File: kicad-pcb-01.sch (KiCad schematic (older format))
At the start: 24 parts, among them SW1 SW_Push, U1 ATmega32U4-AU, Y1 16MHz

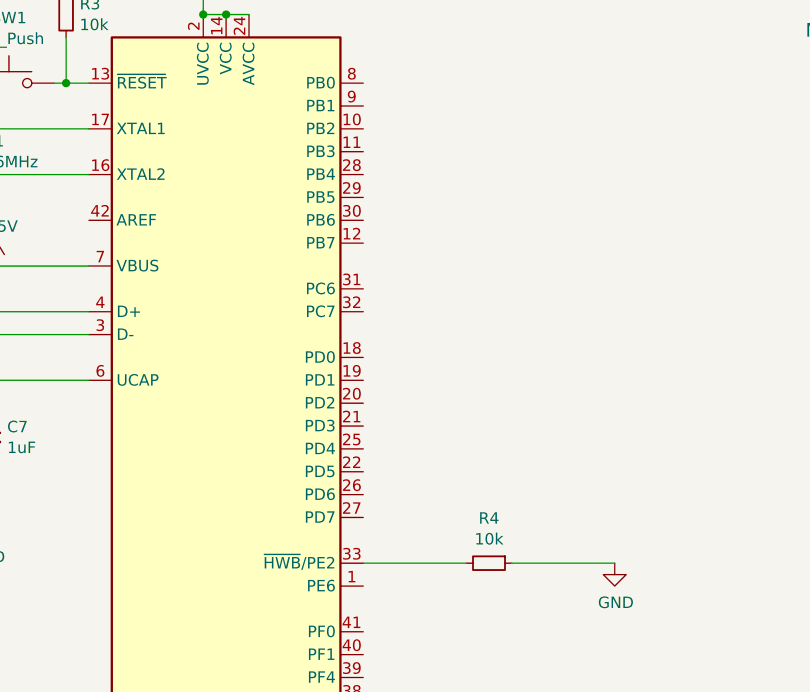
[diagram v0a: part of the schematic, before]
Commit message: routing complete
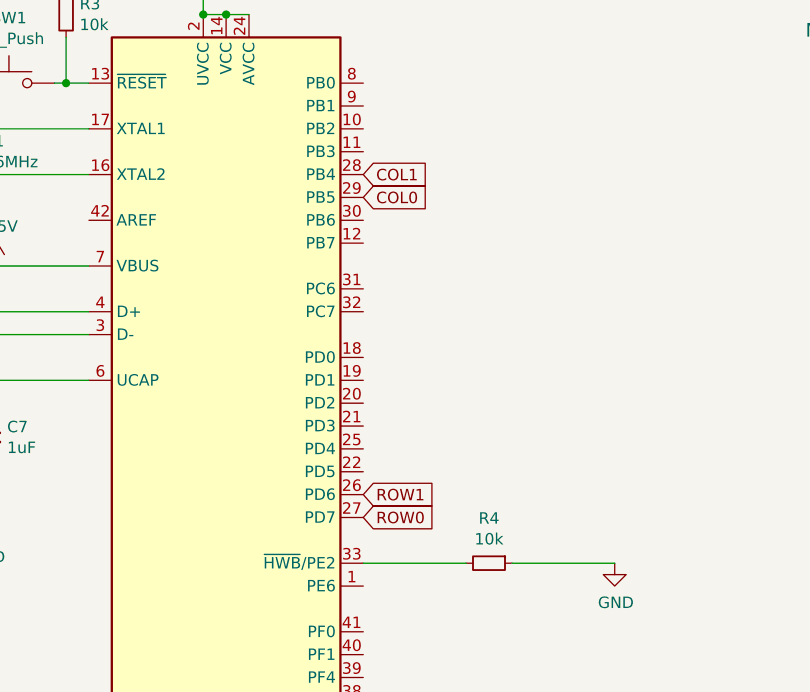
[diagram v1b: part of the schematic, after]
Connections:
- net COL0: now also U1.29 (PB5)
- net COL1: now also U1.28 (PB4)
- net ROW0: now also U1.27 (PD7)
- net ROW1: now also U1.26 (PD6)
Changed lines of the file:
@@
 Text GLabel 8050 2500 1    50   Input ~ 0
 COL1
+Text GLabel 4050 3150 2    50   Input ~ 0
+ROW1
+Text GLabel 4050 3250 2    50   Input ~ 0
+ROW0
+Text GLabel 4050 1750 2    50   Input ~ 0
+COL1
+Text GLabel 4050 1850 2    50   Input ~ 0
+COL0
 $EndSCHEMATC

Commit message: added lcsc part ref:
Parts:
- C1, C2, C3: LCSC (none) -> C1711
- C4, C5: LCSC (none) -> C465168
- C6: LCSC (none) -> C307520
- C7: LCSC (none) -> C116352
- D1, D2, D3, D4: LCSC (none) -> C77978
- F1: LCSC (none) -> C151162
- R1, R2: LCSC (none) -> C413152
- R3, R4: LCSC (none) -> C191101
- SW1: LCSC (none) -> C221929
- U1: LCSC (none) -> C44854
- USB1: LCSC (none) -> C105424
- Y1: LCSC (none) -> C254367
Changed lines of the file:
@@
 F 2 "Package_QFP:TQFP-44_10x10mm_P0.8mm" H 3450 2850 50  0001 C CIN
 F 3 "http://ww1.microchip.com/downloads/en/DeviceDoc/Atmel-7766-8-bit-AVR-ATmega16U4-32U4_Datasheet.pdf" H 3450 2850 50  0001 C CNN
+F 4 "C44854" H 3450 2850 50  0001 C CNN "LCSC"
 	1    3450 2850
 	1    0    0    -1
@@
 F 2 "Resistor_SMD:R_0805_2012Metric" H 4600 3450 50  0001 C CNN
 F 3 "~" H 4600 3450 50  0001 C CNN
+F 4 "C191101" V 4600 3450 50  0001 C CNN "LCSC"
 	1    4600 3450
 	0    1    1    0
@@
 F 2 "Resistor_SMD:R_0805_2012Metric" H 2300 2350 50  0001 C CNN
 F 3 "~" H 2300 2350 50  0001 C CNN
+F 4 "C413152" V 2300 2350 50  0001 C CNN "LCSC"
 	1    2300 2350
 	0    1    1    0
@@
 F 2 "Resistor_SMD:R_0805_2012Metric" H 2000 2450 50  0001 C CNN
 F 3 "~" H 2000 2450 50  0001 C CNN
+F 4 "C413152" V 2000 2450 50  0001 C CNN "LCSC"
 	1    2000 2450
 	0    1    1    0
@@
 F 2 "Capacitor_SMD:C_0805_2012Metric" H 2400 2900 50  0001 C CNN
 F 3 "~" H 2400 2900 50  0001 C CNN
+F 4 "C116352" H 2400 2900 50  0001 C CNN "LCSC"
 	1    2400 2900
 	1    0    0    -1
@@
 F 2 "Capacitor_SMD:C_0805_2012Metric" H 850 4050 50  0001 C CNN
 F 3 "~" H 850 4050 50  0001 C CNN
+F 4 "C1711" H 850 4050 50  0001 C CNN "LCSC"
 	1    850  4050
 	1    0    0    -1
@@
 F 2 "Capacitor_SMD:C_0805_2012Metric" H 1300 4050 50  0001 C CNN
 F 3 "~" H 1300 4050 50  0001 C CNN
+F 4 "C1711" H 1300 4050 50  0001 C CNN "LCSC"
 	1    1300 4050
 	1    0    0    -1
@@
 F 2 "Capacitor_SMD:C_0805_2012Metric" H 1700 4050 50  0001 C CNN
 F 3 "~" H 1700 4050 50  0001 C CNN
+F 4 "C1711" H 1700 4050 50  0001 C CNN "LCSC"
 	1    1700 4050
 	1    0    0    -1
@@
 F 2 "Capacitor_SMD:C_0805_2012Metric" H 2100 4050 50  0001 C CNN
 F 3 "~" H 2100 4050 50  0001 C CNN
+F 4 "C307520" H 2100 4050 50  0001 C CNN "LCSC"
 	1    2100 4050
 	1    0    0    -1
@@
 F 2 "Crystal:Crystal_SMD_3225-4Pin_3.2x2.5mm" H 2250 1650 50  0001 C CNN
 F 3 "~" H 2250 1650 50  0001 C CNN
+F 4 "C254367" V 2250 1650 50  0001 C CNN "LCSC"
 	1    2250 1650
 	0    1    1    0
@@
 F 2 "Capacitor_SMD:C_0805_2012Metric" H 1950 1400 50  0001 C CNN
 F 3 "~" H 1950 1400 50  0001 C CNN
+F 4 "C465168" V 1950 1400 50  0001 C CNN "LCSC"
 	1    1950 1400
 	0    1    1    0
@@
 F 2 "Capacitor_SMD:C_0805_2012Metric" H 1950 1850 50  0001 C CNN
 F 3 "~" H 1950 1850 50  0001 C CNN
+F 4 "C465168" V 1950 1850 50  0001 C CNN "LCSC"
 	1    1950 1850
 	0    1    1    0
@@
 F 2 "random-keyboard-parts:SKQG-1155865" H 2500 1550 50  0001 C CNN
 F 3 "~" H 2500 1550 50  0001 C CNN
+F 4 "C221929" H 2500 1350 50  0001 C CNN "LCSC"
 	1    2500 1350
 	1    0    0    -1
@@
 F 2 "Resistor_SMD:R_0805_2012Metric" H 2750 1050 50  0001 C CNN
 F 3 "~" H 2750 1050 50  0001 C CNN
+F 4 "C191101" H 2750 1050 50  0001 C CNN "LCSC"
 	1    2750 1050
 	1    0    0    -1
@@
 F 2 "random-keyboard-parts:Molex-0548190589" H 6350 1550 60  0001 C CNN
 F 3 "" H 6350 1550 60  0001 C CNN
+F 4 "C105424" V 6350 1550 50  0001 C CNN "LCSC"
 	1    6350 1550
 	0    -1   -1   0
@@
 F 2 "Fuse:Fuse_1206_3216Metric" H 7950 1150 50  0001 L CNN
 F 3 "~" H 7900 1350 50  0001 C CNN
+F 4 "C151162" V 7900 1350 50  0001 C CNN "LCSC"
 	1    7900 1350
 	0    1    1    0
@@
 F 2 "Diode_SMD:D_SOD-123" V 6950 3400 50  0001 C CNN
 F 3 "~" V 6950 3400 50  0001 C CNN
+F 4 "C77978" V 6950 3400 50  0001 C CNN "LCSC"
 	1    6950 3400
 	0    -1   -1   0
@@
 F 2 "Diode_SMD:D_SOD-123" V 7700 3400 50  0001 C CNN
 F 3 "~" V 7700 3400 50  0001 C CNN
+F 4 "C77978" V 7700 3400 50  0001 C CNN "LCSC"
 	1    7700 3400
 	0    -1   -1   0
@@
 F 2 "Diode_SMD:D_SOD-123" V 7700 4250 50  0001 C CNN
 F 3 "~" V 7700 4250 50  0001 C CNN
+F 4 "C77978" V 7700 4250 50  0001 C CNN "LCSC"
 	1    7700 4250
 	0    -1   -1   0
@@
 F 2 "Diode_SMD:D_SOD-123" V 6950 4250 50  0001 C CNN
 F 3 "~" V 6950 4250 50  0001 C CNN
+F 4 "C77978" V 6950 4250 50  0001 C CNN "LCSC"
 	1    6950 4250
 	0    -1   -1   0
